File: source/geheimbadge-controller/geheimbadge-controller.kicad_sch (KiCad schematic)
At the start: 1 part, among them J1 SAOv2

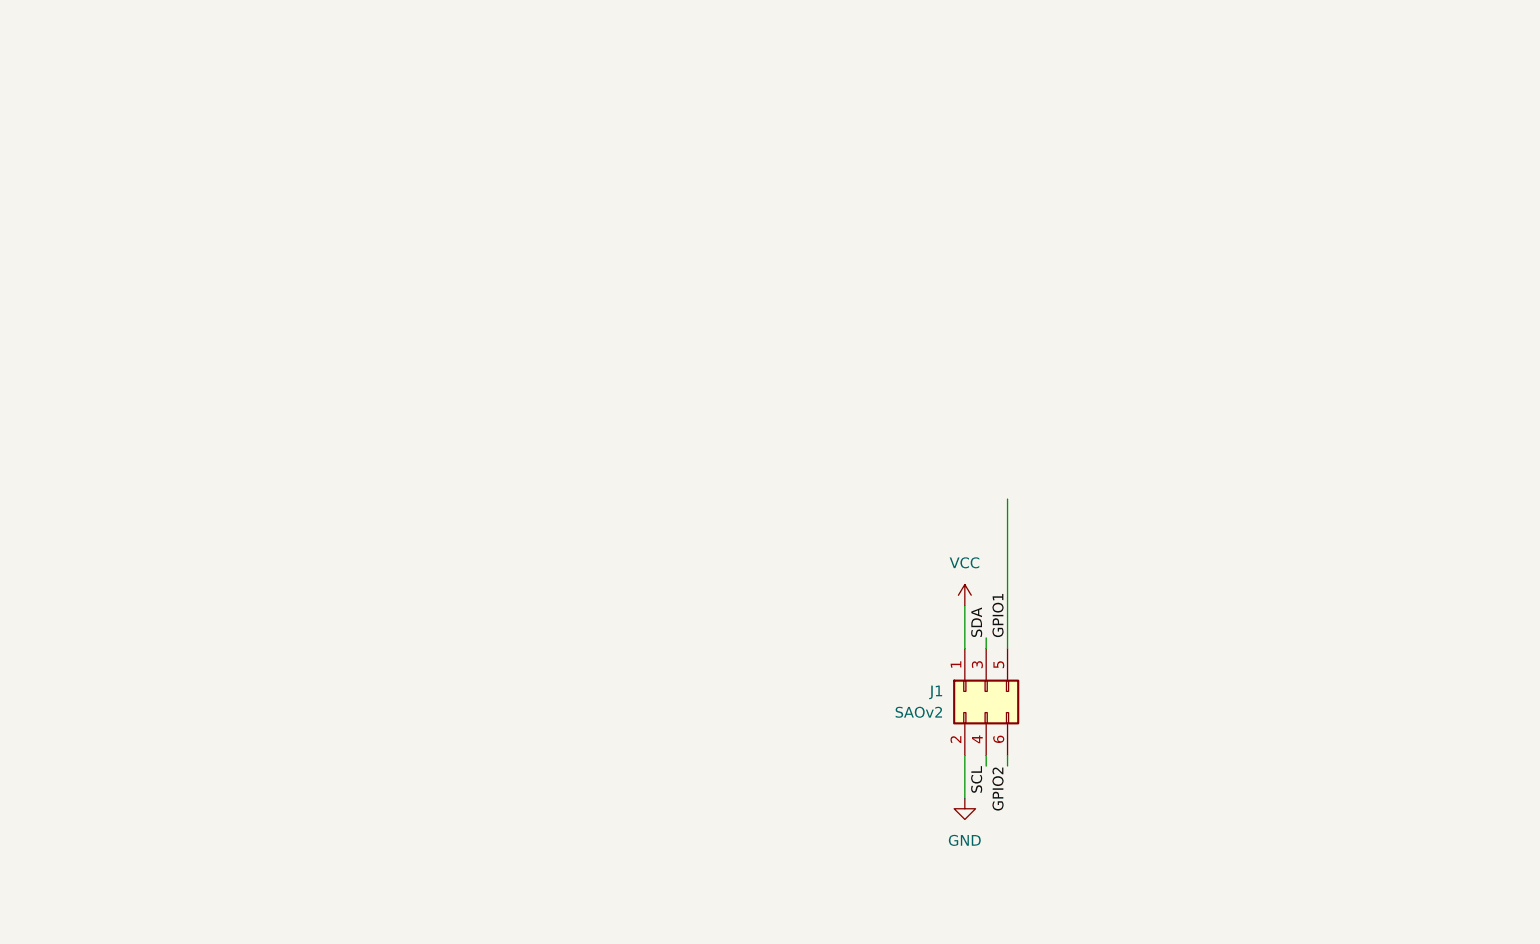
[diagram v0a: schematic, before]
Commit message: finalized controller design
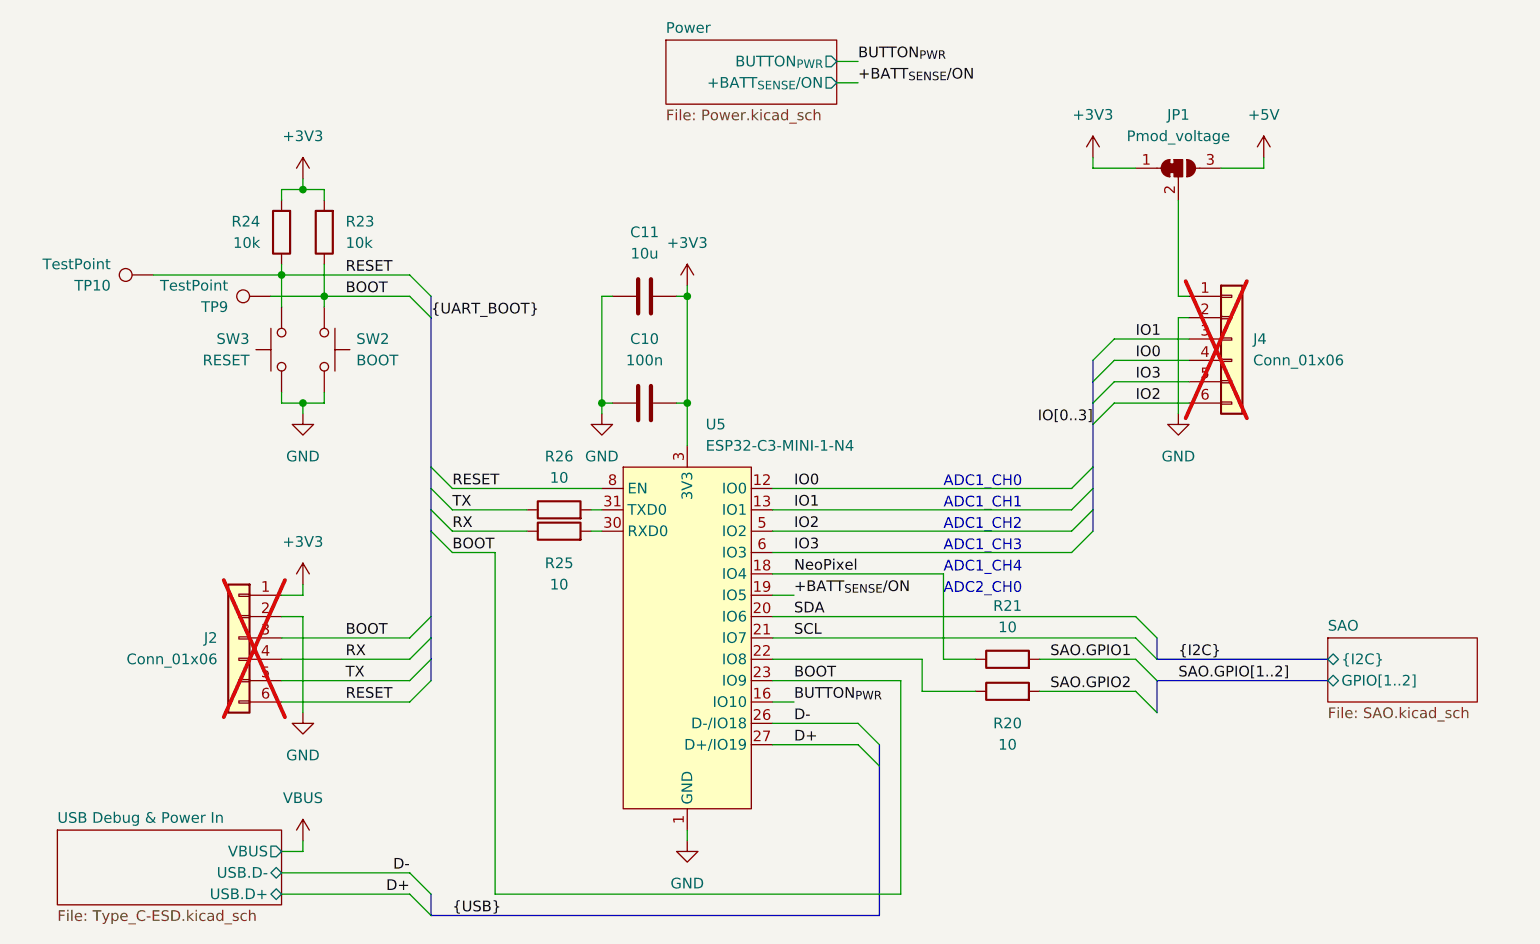
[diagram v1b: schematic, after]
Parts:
- removed J1: SAOv2, Connector_PinSocket_2.54mm:PinSocket_2x03_P2.54mm_Vertical, symbol Connector_Generic:Conn_02x03_Odd_Even
- added C10: 100n, Capacitor_SMD:C_0603_1608Metric, symbol Device:C
- added C11: 10u, Capacitor_SMD:C_0805_2012Metric, symbol Device:C
- added J2, J4: Conn_01x06, Connector_PinSocket_2.54mm:PinSocket_1x06_P2.54mm_Horizontal, symbol Connector_Generic:Conn_01x06
- added JP1: Pmod_voltage, Jumper:SolderJumper-3_P1.3mm_Bridged12_RoundedPad1.0x1.5mm, symbol Jumper:SolderJumper_3_Bridged12
- added R20, R21, R25, R26: 10, Resistor_SMD:R_0603_1608Metric, symbol Device:R
- added R23, R24: 10k, Resistor_SMD:R_0603_1608Metric, symbol Device:R
- added SW2: BOOT, Button_Switch_SMD:SW_Push_1P1T_XKB_TS-1187A, symbol Switch:SW_Push
- added SW3: RESET, Button_Switch_SMD:SW_Push_1P1T_XKB_TS-1187A, symbol Switch:SW_Push
- added TP10, TP9: TestPoint, TestPoint:TestPoint_Pad_D1.0mm, symbol Connector:TestPoint
- added U5: ESP32-C3-MINI-1-N4, ESP32-C3-MINI:WIFIM-SMD_ESP32-C3-MINI-1, symbol ESP32-C3-MINI:ESP32-C3-MINI-1-N4
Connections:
- net GND: now also C10.2, C11.2, J2.2 (Pin_2), J4.2 (Pin_2), SW2.1, SW3.1, U5.1 (GND), U5.11 (GND), U5.14 (GND), U5.2 (GND), U5.36 (GND), U5.37 (GND), U5.38 (GND), U5.39 (GND), U5.40 (GND), U5.41 (GND), U5.42 (GND), U5.43 (GND), U5.44 (GND), U5.45 (GND), U5.46 (GND), U5.47 (GND), U5.48 (GND), U5.49 (GND), U5.50 (GND), U5.51 (GND), U5.52 (GND), U5.53 (GND)
- net SCL: now also U5.21 (IO7)
- net SDA: now also U5.20 (IO6)
- new net: R20.1, U5.22 (IO8)
- new net: J4.1 (Pin_1), JP1.2 (C)
- new net: R25.2, U5.30 (RXD0)
- new net: U5.10 (NC), U5.15 (NC), U5.17 (NC), U5.24 (NC), U5.25 (NC), U5.28 (NC), U5.29 (NC), U5.32 (NC), U5.33 (NC), U5.34 (NC), U5.35 (NC), U5.4 (NC), U5.7 (NC), U5.9 (NC)
- new net: R26.2, U5.31 (TXD0)
- new net +3V3: C10.1, C11.1, J2.1 (Pin_1), JP1.1 (A), R23.2, R24.2, U5.3 (3V3)
- new net +5V: JP1.3 (B)
- new net +BATT_{SENSE}/ON: U5.19 (IO5)
- new net BOOT: J2.3 (Pin_3), R23.1, SW2.2, TP9.1, U5.23 (IO9)
- new net BUTTON_{PWR}: U5.16 (IO10)
- new net D+: U5.27 (D+/IO19)
- new net D-: U5.26 (D-/IO18)
- new net IO0: J4.4 (Pin_4), U5.12 (IO0)
- new net IO1: J4.3 (Pin_3), U5.13 (IO1)
- new net IO2: J4.6 (Pin_6), U5.5 (IO2)
- new net IO3: J4.5 (Pin_5), U5.6 (IO3)
- new net NeoPixel: R21.1, U5.18 (IO4)
- new net RESET: J2.6 (Pin_6), R24.1, SW3.2, TP10.1, U5.8 (EN)
- new net RX: J2.4 (Pin_4), R25.1
- new net SAO.GPIO1: R21.2
- new net SAO.GPIO2: R20.2
- new net TX: J2.5 (Pin_5), R26.1
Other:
- added sheet Power (Power.kicad_sch)
- added sheet SAO (SAO.kicad_sch)
- added sheet USB Debug & Power In (Type_C-ESD.kicad_sch)
- note added: "ADC1_CH0"
- note added: "ADC1_CH1"
- note added: "ADC1_CH2"
- note added: "ADC1_CH3"
- note added: "ADC1_CH4"
- note added: "ADC2_CH0"
